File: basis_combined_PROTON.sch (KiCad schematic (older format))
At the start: 192 parts, among them J1 USB_B_Micro, J2 USB_B_Micro, SW1 Rotary_Encoder_Switch, SW2 Rotary_Encoder_Switch, SW3 Rotary_Encoder_Switch, SW4 SW_Push, SW5 SW_Push, U1 ATmega32U4-AU, U2 ATmega32U4-AU, U3 SRV05-4, U4 SRV05-4, U5 SRV05-4, U6 SRV05-4, Y1 Crystal_GND24_Small, Y2 Crystal_GND24_Small

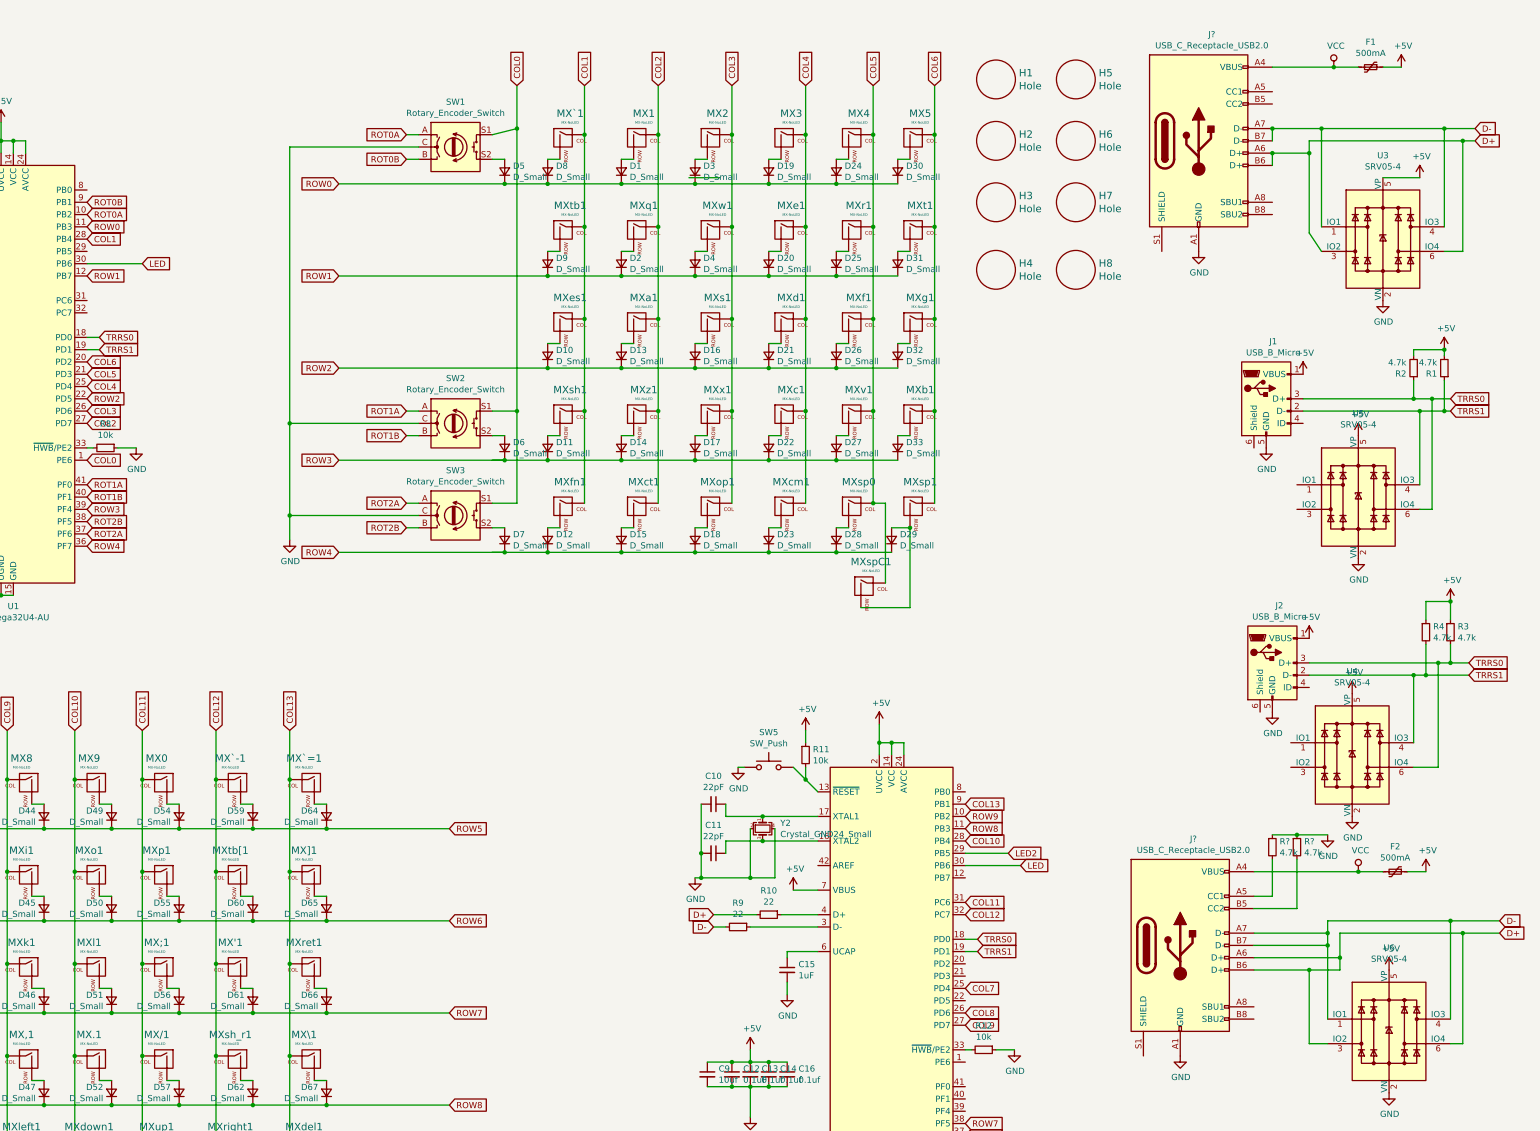
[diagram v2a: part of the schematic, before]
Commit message: checkpoint
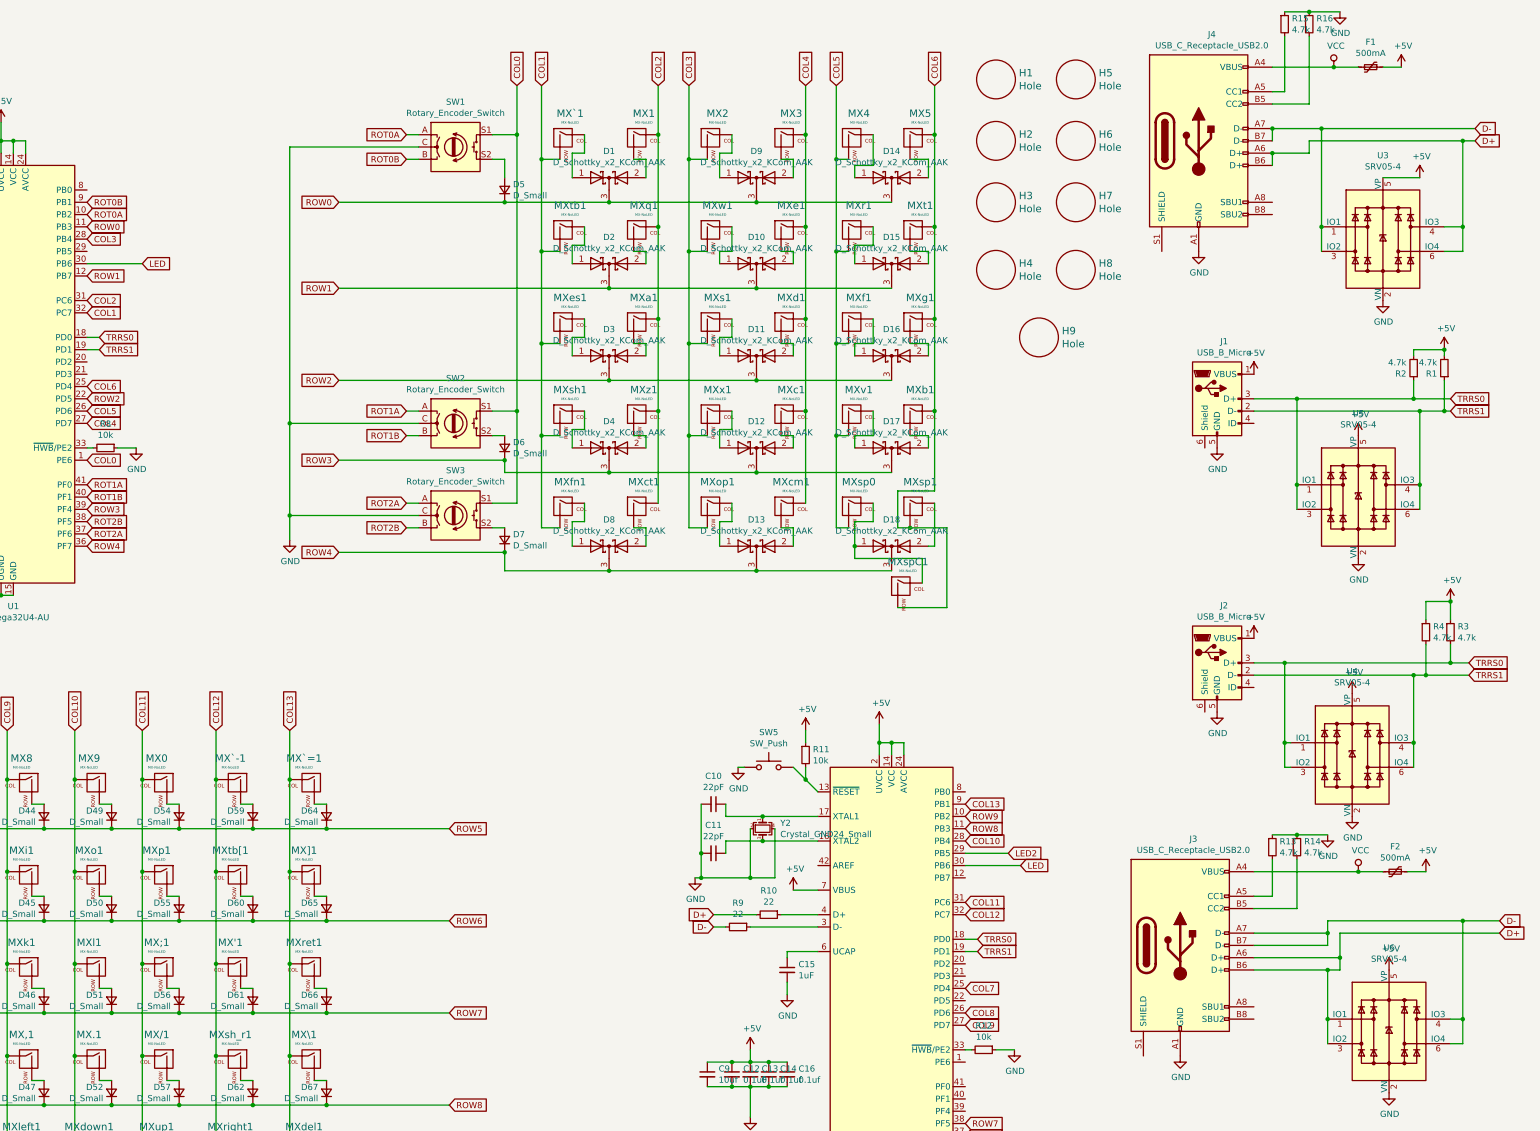
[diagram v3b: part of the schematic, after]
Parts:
- removed D1, D10, D11, D12, D13, D14, D15, D16, D17, D18, D19, D2, D20, D21, D22, D23, D24, D25, D26, D27, D28, D29, D3, D30, D31, D32, D33, D4, D8, D9: D_Small, Diode_SMD:D_SOD-123, symbol Device:D_Small
- added D1, D10, D11, D12, D13, D14, D15, D16, D17, D18, D2, D3, D4, D8, D9: D_Schottky_x2_KCom_AAK, 3d-split-keeb:D_SOT-23_AAK, symbol Device:D_Schottky_x2_KCom_AAK
- added H9: Hole, Keebio-Parts:MountingHole, symbol keebio:Hole
- added R15, R16: 4.7k, Resistor_SMD:R_0805_2012Metric, symbol Device:R_Small
- J1, J2: footprint Connector_USB:USB_Micro-B_Molex_47346-0001 -> 47642-0001:MOLEX_47642-0001
- J3, J4: renamed from J?; footprint (none) -> random-keyboard-parts:USB_C_Receptacle_Hirose_CX90M-16P
- gave numbers to parts that had none: 2
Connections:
- net COL1: now also MX`1.2 (ROW), MXes1.2 (ROW), MXfn1.2 (ROW), MXsh1.2 (ROW), MXtb1.2 (ROW), U1.32 (PC7); no longer MX`1.1 (COL), MXes1.1 (COL), MXfn1.1 (COL), MXsh1.1 (COL), MXtb1.1 (COL), U1.28 (PB4)
- net COL2: now also U1.31 (PC6); no longer U1.27 (PD7)
- net COL3: now also MX2.2 (ROW), MXop1.2 (ROW), MXs1.2 (ROW), MXw1.2 (ROW), MXx1.2 (ROW), U1.28 (PB4); no longer MX2.1 (COL), MXop1.1 (COL), MXs1.1 (COL), MXw1.1 (COL), MXx1.1 (COL), U1.26 (PD6)
- net COL4: now also U1.27 (PD7); no longer U1.25 (PD4)
- net COL5: now also MX4.2 (ROW), MXf1.2 (ROW), MXr1.2 (ROW), MXsp0.2 (ROW), MXv1.2 (ROW), U1.26 (PD6); no longer MX4.1 (COL), MXf1.1 (COL), MXr1.1 (COL), MXsp0.1 (COL), MXspC1.1 (COL), MXv1.1 (COL), U1.21 (PD3)
- net COL6: now also MXsp1.2 (ROW), MXspC1.2 (ROW), U1.25 (PD4); no longer MXsp1.1 (COL), U1.20 (PD2)
- net D+: now also U3.4 (IO3), U6.1 (IO1); no longer U3.3 (IO2), U6.6 (IO4)
- net D-: now also U3.3 (IO2), U6.6 (IO4); no longer U3.4 (IO3), U6.1 (IO1)
- net GND: now also R15.1, R16.1
- net ROW0: now also D1.3 (K), D14.3 (K), D9.3 (K)
- net ROW1: now also D10.3 (K), D15.3 (K), D2.3 (K)
- net ROW2: now also D11.3 (K), D16.3 (K), D3.3 (K)
- net ROW3: now also D12.3 (K), D17.3 (K), D4.3 (K)
- net ROW4: now also D13.3 (K), D18.3 (K), D8.3 (K)
- net TRRS0: now also U4.1 (IO1), U4.3 (IO2), U5.1 (IO1), U5.3 (IO2); no longer U4.6 (IO4), U5.6 (IO4)
- net TRRS1: now also U4.6 (IO4), U5.6 (IO4)
- net at MX1.2 (ROW): now also D1.2 (A)
- net at MXq1.2 (ROW): now also D2.2 (A)
- net at MXa1.2 (ROW): now also D3.2 (A)
- net at MXz1.2 (ROW): now also D4.2 (A)
- net at MXct1.2 (ROW): now also D8.2 (A)
- net at MX3.2 (ROW): now also D9.2 (A)
- net at MXe1.2 (ROW): now also D10.2 (A)
- net at MXd1.2 (ROW): now also D11.2 (A)
- net at MXc1.2 (ROW): now also D12.2 (A)
- net at MXcm1.2 (ROW): now also D13.2 (A)
- net at MX5.2 (ROW): now also D14.2 (A)
- net at MXt1.2 (ROW): now also D15.2 (A)
- net at MXg1.2 (ROW): now also D16.2 (A)
- net at MXb1.2 (ROW): now also D17.2 (A)
- net at J4.A5 (CC1): now also R15.2
- net at J4.B5 (CC2): now also R16.2
- new net: D9.1 (A), MX2.1 (COL)
- new net: D10.1 (A), MXw1.1 (COL)
- new net: D11.1 (A), MXs1.1 (COL)
- new net: D12.1 (A), MXx1.1 (COL)
- new net: D13.1 (A), MXop1.1 (COL)
- new net: D14.1 (A), MX4.1 (COL)
- new net: D15.1 (A), MXr1.1 (COL)
- new net: D16.1 (A), MXf1.1 (COL)
- new net: D17.1 (A), MXv1.1 (COL)
- new net: D18.1 (A), MXsp0.1 (COL), MXspC1.1 (COL)
- new net: D18.2 (A), MXsp1.1 (COL)
- new net: D1.1 (A), MX`1.1 (COL)
- new net: D2.1 (A), MXtb1.1 (COL)
- new net: D3.1 (A), MXes1.1 (COL)
- new net: D4.1 (A), MXsh1.1 (COL)
- new net: D8.1 (A), MXfn1.1 (COL)
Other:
- moved on the sheet: D5, J1, J2, MXspC1

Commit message: Yeah
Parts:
- removed D34, D35, D36, D37, D38, D39, D40, D41, D42, D43, D44, D45, D46, D47, D48, D49, D50, D51, D52, D53, D54, D55, D56, D57, D58, D59, D60, D61, D62, D63: D_Small, Diode_SMD:D_SOD-123, symbol Device:D_Small
- removed H2, H6: Hole, Keebio-Parts:MountingHole, symbol keebio:Hole
- removed R10, R9: 22, Resistor_SMD:R_0805_2012Metric, symbol Device:R_Small
- removed R11, R12: 10k, Resistor_SMD:R_0805_2012Metric, symbol Device:R_Small
- removed SW5: SW_Push, random-keyboard-parts:SKQG-1155865, symbol Switch:SW_Push
- removed U1, U2: ATmega32U4-AU, Package_QFP:TQFP-44_10x10mm_P0.8mm, symbol MCU_Microchip_ATmega:ATmega32U4-AU
- removed U3, U6: SRV05-4, Package_TO_SOT_SMD:SOT-23-6, symbol Power_Protection:SRV05-4
- removed Y1, Y2: Crystal_GND24_Small, Crystal:Crystal_SMD_3225-4Pin_3.2x2.5mm, symbol Device:Crystal_GND24_Small
- added B1, B2: BLUENRG-M2SA, 3d-split-keeb:BLUENRG-M2SA, symbol random-keyboard-parts:BLUENRG-M2SA
- added C17, C19, C21: 4.7uF, Capacitor_SMD:C_0402_1005Metric, symbol Device:C_Small
- added C18, C22, C24, C26, C29, C30, C31, C32, C33, C34, C35, C36, C37, C38: 100nF, Capacitor_SMD:C_0402_1005Metric, symbol Device:C_Small
- added C20, C25: 10nF, Capacitor_SMD:C_0402_1005Metric, symbol Device:C_Small
- added C23, C27, C28: 1uF, Capacitor_SMD:C_0402_1005Metric, symbol Device:C_Small
- added C39, C43: 10uF, Capacitor_SMD:C_0402_1005Metric, symbol Device:C_Small
- added C40, C44: 50uF, Capacitor_SMD:C_0402_1005Metric, symbol Device:C_Small
- added C41, C45: 50nF, Capacitor_SMD:C_0402_1005Metric, symbol Device:C_Small
- added C42, C46: 250uF, Capacitor_SMD:C_0402_1005Metric, symbol Device:C_Small
- added D19, D21: 1N4148, Diode_SMD:D_SOD-123, symbol Diode:1N4148
- added D20, D22: D_Schottky_Small, Diode_SMD:D_SOD-123, symbol Device:D_Schottky_Small
- added D23, D24, D25, D26, D27, D28, D29, D30, D31, D32, D33, D69, D70, D71: WS2812B, LED_SMD:LED_WS2812B_PLCC4_5.0x5.0mm_P3.2mm, symbol LED:WS2812B
- added D34, D35, D36, D37, D38, D39, D40, D41, D42, D43, D44, D45, D46, D47, D48: D_Schottky_x2_KCom_AAK, 3d-split-keeb:D_SOT-23_AAK, symbol Device:D_Schottky_x2_KCom_AAK
- added H10: Hole, 3d-split-keeb:Mounting_Wuerth_WA-SMSI-M2_H3.5mm_9774035243, symbol keebio:Hole
- added J5, J6, J7, J8: FTSH-105-01-L-DV-K, FTSH-105-01-L-DV-K:SAMTEC_FTSH-105-01-L-DV-K, symbol FTSH-105-01-L-DV-K:FTSH-105-01-L-DV-K
- added LS1, LS2: Speaker, 3d-split-keeb:cms-151103-16sp, symbol Device:Speaker
- added Q1, Q2: DTC123J, Package_TO_SOT_SMD:SOT-723, symbol Transistor_BJT:DTC123J
- added R17: 100k, Resistor_SMD:R_0402_1005Metric, symbol Device:R_Small
- added R18: 1M, Resistor_SMD:R_0402_1005Metric, symbol Device:R_Small
- added SW6: SW_Push, random-keyboard-parts:SKQG-1155865, symbol Switch:SW_Push
- added U1, U8: SN74LVC1G07DCK3, SN74LVC1G07DCKR:SN74LVC1G07DCK3, symbol SN74LVC1G07DCKR:SN74LVC1G07DCK3
- added U10, U7: STM32F072CBUx, Package_DFN_QFN:QFN-48-1EP_7x7mm_P0.5mm_EP5.6x5.6mm, symbol MCU_ST_STM32F0:STM32F072CBUx
- added U11, U12: USBLC6-2SC6, Package_TO_SOT_SMD:SOT-666, symbol Power_Protection:USBLC6-2SC6
- added U2, U9: XC6206PxxxMR, Package_TO_SOT_SMD:SOT-23, symbol Regulator_Linear:XC6206PxxxMR
- added U3, U6: LM386, Package_SO:SOIC-8_3.9x4.9mm_P1.27mm, symbol Amplifier_Audio:LM386
- C1: value 10uf -> 4.7uF; footprint Capacitor_SMD:C_0805_2012Metric -> Capacitor_SMD:C_0402_1005Metric
- C10, C2: value 22pF -> 100nF; footprint Capacitor_SMD:C_0805_2012Metric -> Capacitor_SMD:C_0402_1005Metric
- C11, C3: value 22pF -> 4.7uF; footprint Capacitor_SMD:C_0805_2012Metric -> Capacitor_SMD:C_0402_1005Metric
- C12: value 0.1uF -> 1uF; footprint Capacitor_SMD:C_0805_2012Metric -> Capacitor_SMD:C_0402_1005Metric
- C13, C14, C16, C6: value 0.1uf -> 100nF; footprint Capacitor_SMD:C_0805_2012Metric -> Capacitor_SMD:C_0402_1005Metric
- C15: value 1uF -> 100nF; footprint Capacitor_SMD:C_0805_2012Metric -> Capacitor_SMD:C_0402_1005Metric
- C4: value 0.1uF -> 100nF; footprint Capacitor_SMD:C_0805_2012Metric -> Capacitor_SMD:C_0402_1005Metric
- C5: value 0.1uf -> 1uF; footprint Capacitor_SMD:C_0805_2012Metric -> Capacitor_SMD:C_0402_1005Metric
- C7: footprint Capacitor_SMD:C_0805_2012Metric -> Capacitor_SMD:C_0402_1005Metric
- C8: value 0.1uf -> 10nF; footprint Capacitor_SMD:C_0805_2012Metric -> Capacitor_SMD:C_0402_1005Metric
- C9: value 10uf -> 10nF; footprint Capacitor_SMD:C_0805_2012Metric -> Capacitor_SMD:C_0402_1005Metric
- H1, H3, H4, H5, H7, H8, H9: footprint Keebio-Parts:MountingHole -> 3d-split-keeb:Mounting_Wuerth_WA-SMSI-M2_H3.5mm_9774035243
- R1: value 4.7k -> 1M; footprint Resistor_SMD:R_0805_2012Metric -> Resistor_SMD:R_0402_1005Metric
- R13, R14, R15, R16, R2, R3: footprint Resistor_SMD:R_0805_2012Metric -> Resistor_SMD:R_0402_1005Metric
- R4: value 4.7k -> 100k; footprint Resistor_SMD:R_0805_2012Metric -> Resistor_SMD:R_0402_1005Metric
- R5: value 22 -> 1.2k; footprint Resistor_SMD:R_0805_2012Metric -> Resistor_SMD:R_0402_1005Metric
- R6: value 22 -> 10; footprint Resistor_SMD:R_0805_2012Metric -> Resistor_SMD:R_0402_1005Metric
- R7: value 10k -> 1.2k; footprint Resistor_SMD:R_0805_2012Metric -> Resistor_SMD:R_0402_1005Metric
- R8: value 10k -> 10; footprint Resistor_SMD:R_0805_2012Metric -> Resistor_SMD:R_0402_1005Metric
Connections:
- net +5V: now also C15.1, C7.1, R1.1, C27.1, C29.1, C30.1, C31.1, C32.1, C33.1, C34.1, C35.1, C36.1, C37.1, C38.1, D20.1 (K), D22.1 (K), D23.1 (VDD), D24.1 (VDD), D25.1 (VDD), D26.1 (VDD), D27.1 (VDD), D28.1 (VDD), D29.1 (VDD), D30.1 (VDD), D31.1 (VDD), D32.1 (VDD), D33.1 (VDD), D69.1 (VDD), D70.1 (VDD), D71.1 (VDD), R18.1, U1.5 (VCC), U2.3 (VI), U3.6 (V+), U6.6 (V+), U8.5 (VCC), U9.3 (VI); no longer C1.1, C12.1, C4.1, C5.1, C6.1, C8.1, C9.1, R1.2, R2.2, R3.1, R4.1, R7.1
- net COL0: now also U7.28 (PB15)
- net COL1: now also U7.46 (PB9)
- net COL10: now also U10.26 (PB13)
- net COL11: now also MX/1.2 (ROW), MX0.2 (ROW), MX;1.2 (ROW), MXp1.2 (ROW), MXup1.2 (ROW), U10.27 (PB14); no longer MX/1.1 (COL), MX0.1 (COL), MX;1.1 (COL), MXp1.1 (COL), MXup1.1 (COL)
- net COL12: now also U10.28 (PB15)
- net COL13: now also U10.40 (PB4)
- net COL2: now also U7.43 (PB7)
- net COL3: now also U7.42 (PB6)
- net COL4: now also U7.41 (PB5)
- net COL5: now also U7.40 (PB4)
- net COL6: now also U7.39 (PB3)
- net COL7: now also MX6.2 (ROW), MXh1.2 (ROW), MXn1.2 (ROW), MXy1.2 (ROW), U10.18 (PB0); no longer MX6.1 (COL), MXh1.1 (COL), MXn1.1 (COL), MXy1.1 (COL)
- net COL8: now also U10.19 (PB1)
- net COL9: now also MX,1.2 (ROW), MX8.2 (ROW), MXi1.2 (ROW), MXk1.2 (ROW), MXleft1.2 (ROW), U10.20 (PB2); no longer MX,1.1 (COL), MX8.1 (COL), MXi1.1 (COL), MXk1.1 (COL), MXleft1.1 (COL)
- net D+: now also U10.33 (PA12), U11.3 (IO2), U11.4 (IO2), U12.3 (IO2), U12.4 (IO2), U7.33 (PA12); no longer R6.2
- net D-: now also U10.32 (PA11), U11.1 (IO1), U11.6 (IO1), U12.1 (IO1), U12.6 (IO1), U7.32 (PA11); no longer R5.2
- net GND: now also R1.2, R4.2, B1.21 (GND), B1.8 (GND), B2.21 (GND), B2.8 (GND), C17.2, C18.2, C19.2, C20.2, C21.2, C22.2, C23.2, C24.2, C25.2, C26.2, C27.2, C28.2, C29.2, C30.2, C31.2, C32.2, C33.2, C34.2, C35.2, C36.2, C37.2, C38.2, C40.1, C41.1, C44.1, C45.1, D23.3 (VSS), D24.3 (VSS), D25.3 (VSS), D26.3 (VSS), D27.3 (VSS), D28.3 (VSS), D29.3 (VSS), D30.3 (VSS), D31.3 (VSS), D32.3 (VSS), D33.3 (VSS), D69.3 (VSS), D70.3 (VSS), D71.3 (VSS), J5.3, J5.5, J5.9, J6.3, J6.5, J6.9, J7.3, J7.5, J7.9, J8.3, J8.5, J8.9, LS1.2, LS2.2, Q1.2 (E), Q2.2 (E), R17.2, R18.2, U1.3 (GND), U10.23 (VSS), U10.35 (VSS), U10.47 (VSS), U10.49 (VSS), U10.8 (VSSA), U11.2 (GND), U12.2 (GND), U2.1 (GND), U3.2 (-), U3.4 (GND), U6.2 (-), U6.4 (GND), U7.23 (VSS), U7.35 (VSS), U7.47 (VSS), U7.49 (VSS), U7.8 (VSSA), U8.3 (GND), U9.1 (GND); no longer R8.1, SW4.1
- net ROT0A: now also U7.31 (PA10)
- net ROT0B: now also U7.29 (PA8)
- net ROT1A: now also U7.26 (PB13)
- net ROT1B: now also U7.27 (PB14)
- net ROT2A: now also U7.22 (PB11)
- net ROT2B: now also U7.25 (PB12)
- net ROW0: now also U7.38 (PA15); no longer D5.1 (K)
- net ROW1: now also U7.5 (PF0)
- net ROW2: now also D5.1 (K), U7.19 (PB1)
- net ROW3: now also U7.20 (PB2)
- net ROW4: now also U7.21 (PB10)
- net ROW5: now also D34.3 (K), D39.3 (K), D44.3 (K), U10.31 (PA10)
- net ROW6: now also D35.3 (K), D40.3 (K), D45.3 (K), U10.29 (PA8)
- net ROW7: now also D36.3 (K), D41.3 (K), D46.3 (K), U10.25 (PB12)
- net ROW8: now also D37.3 (K), D42.3 (K), D47.3 (K), U10.41 (PB5)
- net ROW9: now also D38.3 (K), D43.3 (K), D48.3 (K), U10.43 (PB7)
- net VCC: now also U11.5 (VBUS), U12.5 (VBUS)
- net at R8.2: now also C45.2
- net at R6.1: now also C42.2, U3.5
- net at R5.1: now also U3.1 (GAIN)
- net at MX9.2 (ROW): now also D39.2 (A)
- net at MXo1.2 (ROW): now also D40.2 (A)
- net at MXl1.2 (ROW): now also D41.2 (A)
- net at MX.1.2 (ROW): now also D42.2 (A)
- net at MXdown1.2 (ROW): now also D43.2 (A)
- net at MX7.2 (ROW): now also D34.2 (A)
- net at MXu1.2 (ROW): now also D35.2 (A)
- net at MXj1.2 (ROW): now also D36.2 (A)
- net at MXm1.2 (ROW): now also D37.2 (A)
- net at MXsp_r1.2 (ROW), MXsp_rC1.2 (ROW): now also D38.2 (A)
- net at MXsp_r0.2 (ROW): now also D38.1 (A)
- net at MX`-1.2 (ROW): now also D44.2 (A)
- net at MXtb[1.2 (ROW): now also D45.2 (A)
- net at MX'1.2 (ROW): now also D46.2 (A)
- net at MXsh_r1.2 (ROW): now also D47.2 (A)
- net at MXright1.2 (ROW): now also D48.2 (A)
- net +3V3: now reaches C2.1
- net +3V3: now also C1.1, C10.1, C12.1, C3.1, C4.1, C5.1, C6.1, C9.1, J1.3 (D+), J2.3 (D+), R2.2, R3.1, SW4.1, U4.1 (IO1), U4.3 (IO2), U5.1 (IO1), U5.3 (IO2), B1.5 (VIN), B2.5 (VIN), C17.1, C18.1, C19.1, C22.1, C23.1, C24.1, C25.1, C26.1, C28.1, D20.2 (A), D22.2 (A), J5.1, J6.1, J7.1, J8.1, SW6.1, U10.1 (VBAT), U10.24 (VDD), U10.36 (VDDIO2), U10.48 (VDD), U10.9 (VDDA), U2.2 (VO), U7.1 (VBAT), U7.24 (VDD), U7.36 (VDDIO2), U7.48 (VDD), U7.9 (VDDA), U9.2 (VO)
- net at R7.2: now also C43.1; no longer SW4.2
- net NRST: now reaches C11.1
- net NRST: now also C21.1, J5.10, J7.10, Q1.3 (C), Q2.3 (C), U10.7 (NRST), U7.7 (NRST)
- removed net TRRS0: J1.3 (D+), J2.3 (D+), R2.1, R3.2, U4.1 (IO1), U4.3 (IO2), U5.1 (IO1), U5.3 (IO2)
- net TRRS1 renamed usart1
- net usart1: now also R2.1, R3.2, U10.30 (PA9), U7.30 (PA9); no longer R1.1, R4.2
- new net: D44.1 (A), MX0.1 (COL)
- new net: D45.1 (A), MXp1.1 (COL)
- new net: D46.1 (A), MX;1.1 (COL)
- new net: D47.1 (A), MX/1.1 (COL)
- new net: D48.1 (A), MXup1.1 (COL)
- new net: D39.1 (A), MX8.1 (COL)
- new net: D40.1 (A), MXi1.1 (COL)
- new net: D41.1 (A), MXk1.1 (COL)
- new net: D42.1 (A), MX,1.1 (COL)
- new net: D43.1 (A), MXleft1.1 (COL)
- new net: D34.1 (A), MX6.1 (COL)
- new net: D35.1 (A), MXy1.1 (COL)
- new net: D36.1 (A), MXh1.1 (COL)
- new net: D37.1 (A), MXn1.1 (COL)
- new net: B2.19 (RESETN), J6.10
- new net: B1.19 (RESETN), J8.10
- new net: C40.2, U3.7 (BYPASS)
- new net: C39.2, U3.8 (GAIN)
- new net: C42.1, LS1.1
- new net: C41.2, R6.2
- new net: C39.1, R5.2
- new net: R7.1, U6.1 (GAIN)
- new net: C46.2, R8.1, U6.5
- new net: C44.2, U6.7 (BYPASS)
- new net: C43.2, U6.8 (GAIN)
- new net: C46.1, LS2.1
- new net: C20.1, D19.1 (K), R17.1, U7.44 (BOOT0)
- new net: D19.2 (A), Q1.1 (B), SW6.2
- new net: C8.1, D21.1 (K), R4.1, U10.44 (BOOT0)
- new net: D21.2 (A), Q2.1 (B), SW4.2
- new net: D27.2 (DOUT), D29.4 (DIN)
- new net: D29.2 (DOUT), D31.4 (DIN)
- new net: D31.2 (DOUT), D33.4 (DIN)
- new net: D33.2 (DOUT), D69.4 (DIN)
- new net: D69.2 (DOUT), D70.4 (DIN)
- new net: D70.2 (DOUT), D71.4 (DIN)
- new net: D23.2 (DOUT), D24.4 (DIN)
- new net: D24.2 (DOUT), D25.4 (DIN)
- new net: D25.2 (DOUT), D26.4 (DIN)
- new net: D26.2 (DOUT), D28.4 (DIN)
- new net: D28.2 (DOUT), D30.4 (DIN)
- new net: D30.2 (DOUT), D32.4 (DIN)
- new net LED3v: U1.2 (A), U7.45 (PB8)
- new net LED3v3: U10.45 (PB8), U8.2 (A)
- new net LED5V: D23.4 (DIN), D27.4 (DIN), U1.4 (Y), U8.4 (Y)
- new net SPKR2: U10.15 (PA5), U3.3 (+), U6.3 (+), U7.15 (PA5)
- new net SWCLK: B1.12 (DIO9), B2.12 (DIO9), J5.4, J6.4, J7.4, J8.4, U10.37 (PA14), U7.37 (PA14)
- new net SWDIO: B1.13 (DIO10), B2.13 (DIO10), J5.2, J6.2, J7.2, J8.2, U10.34 (PA13), U7.34 (PA13)
- new net USART2_CK: B1.14 (ANATEST1), B2.14 (ANATEST1), U10.14 (PA4), U7.14 (PA4)
- new net USART2_CTS: B1.15 (DIO0), B2.15 (DIO0), U10.10 (PA0), U7.10 (PA0)
- new net USART2_RTS: B1.9 (DIO6), B2.18 (DIO1), B2.9 (DIO6), U10.11 (PA1), U7.11 (PA1)
- new net USART2_RX: B1.10 (DIO8), B2.10 (DIO8), B2.4 (DIO5), U10.13 (PA3), U7.13 (PA3)
- new net USART2_TX: B1.11 (DIO11), B2.11 (DIO11), B2.3 (DIO4), U10.12 (PA2), U7.12 (PA2)
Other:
- moved on the sheet: D5, H3, H4, H7, H8, H9, MX'1, MX.1, MX7, MX9, MX`-1, MXdown1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

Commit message: Add shield grounding, curves etc
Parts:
- added C47, C48: 4.7nF, Capacitor_SMD:C_0402_1005Metric, symbol Device:C_Small
- added C49, C50: 100nF, Capacitor_SMD:C_0402_1005Metric, symbol Device:C_Small
- added H2: Hole, 3d-split-keeb:Mounting_Wuerth_WA-SMSI-M2_H3.5mm_9774035243, symbol keebio:Hole
- added R10, R9: 1M, Resistor_SMD:R_0402_1005Metric, symbol Device:R_Small
- added STAB1, STAB2: Hole, keyswitches:Stabilizer_MX_2u, symbol keebio:Hole
- H1, H10, H7, H8: symbol keebio:Hole -> keebio:eHole
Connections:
- net GND: now also C47.2, C48.2, C49.2, C50.2, R10.2, R9.2
- net USART2_RTS: no longer B2.9 (DIO6)
- net USART2_RX: no longer B2.4 (DIO5)
- net USART2_TX: no longer B2.3 (DIO4)
- net VCC: now also C49.1, C50.1
- net GNDS: now reaches J4.S1 (SHIELD)
- net GNDS: now also H1.1 (PIN), H10.1 (PIN), H7.1 (PIN), H8.1 (PIN), J1.6 (Shield), J2.6 (Shield), J3.S1 (SHIELD), C47.1, C48.1, R10.1, R9.1
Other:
- moved on the sheet: U11, U12
